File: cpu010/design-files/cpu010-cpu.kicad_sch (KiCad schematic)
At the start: 3 parts, among them U201 MC68010P, U202 74ACT163, Y201 40MHz

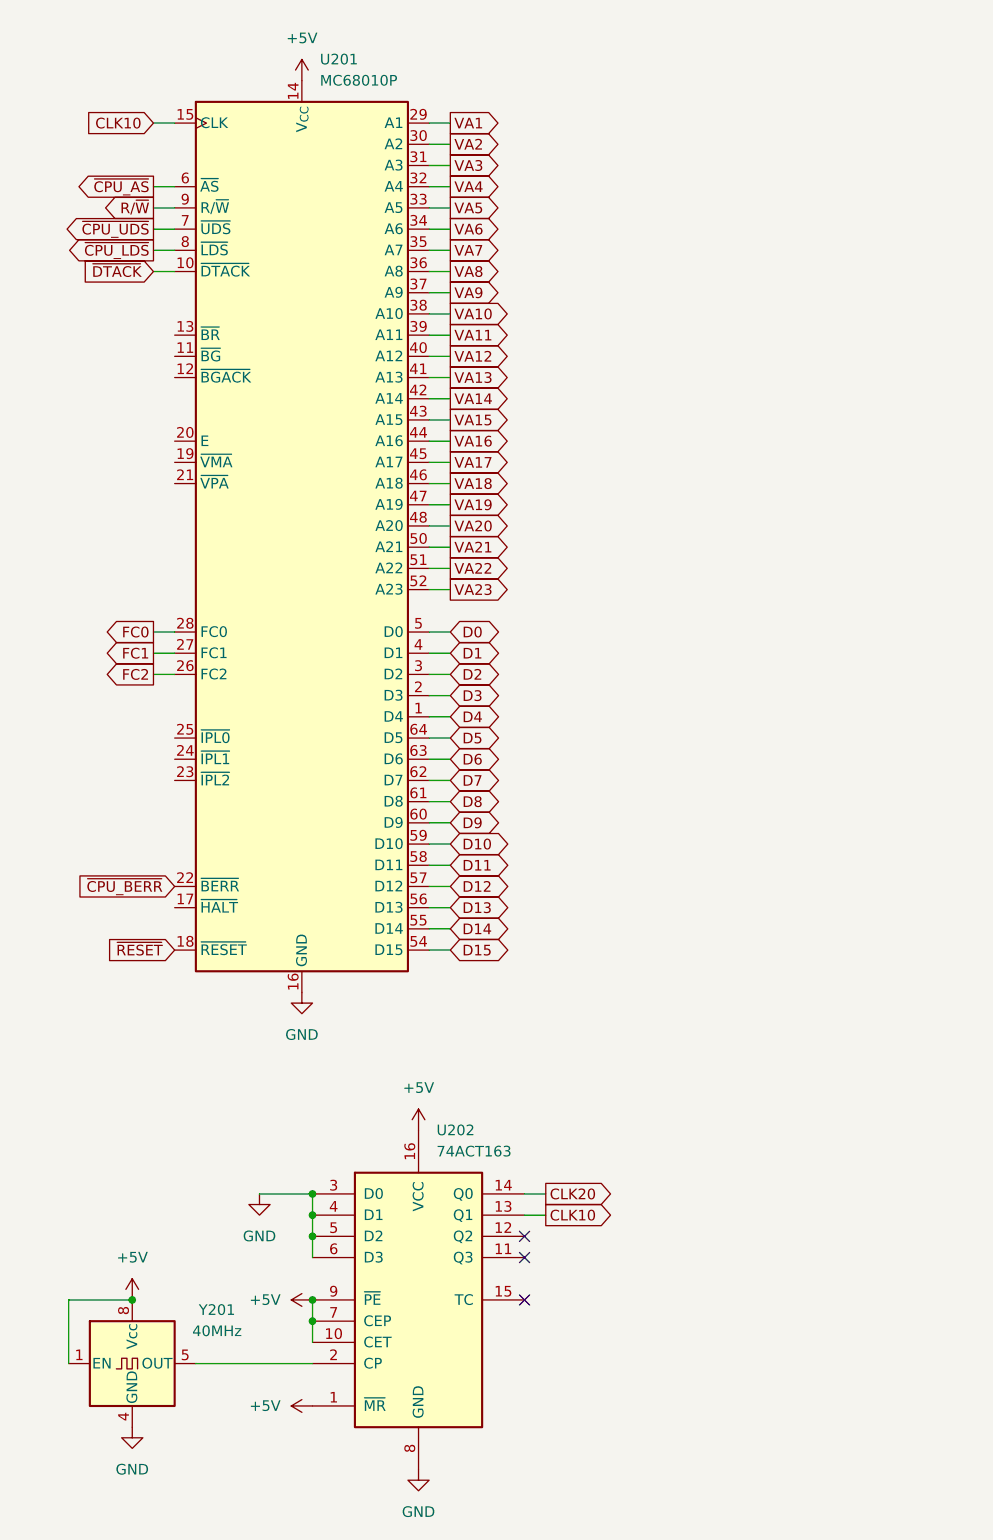
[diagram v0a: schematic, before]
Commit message: Open-drain inverter for DTACKs.
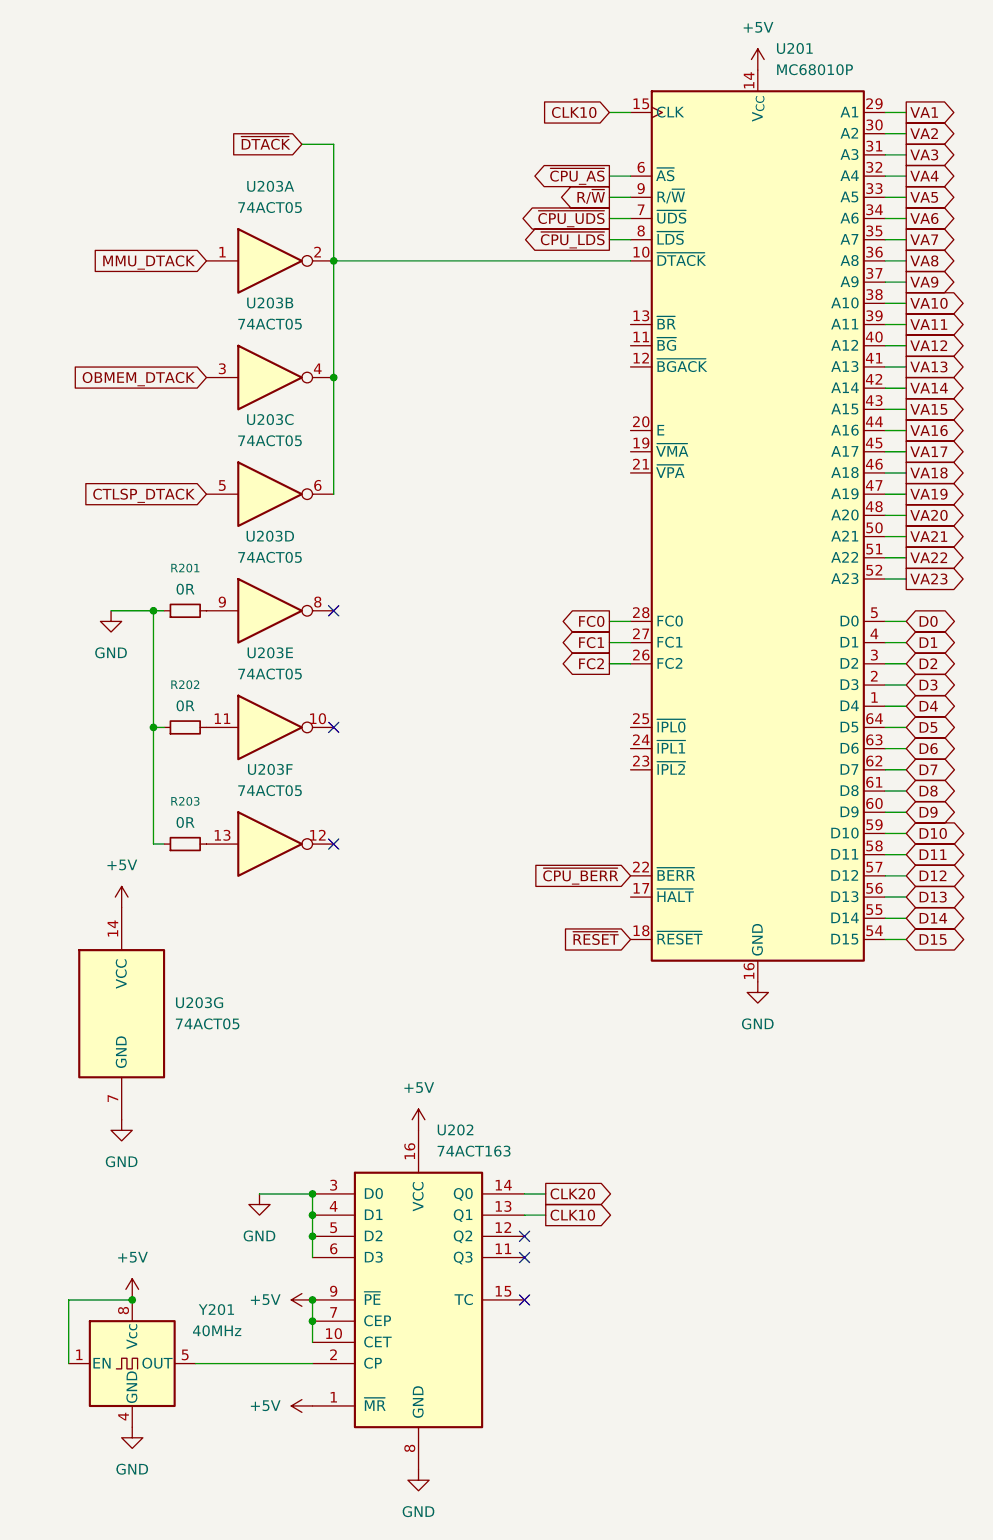
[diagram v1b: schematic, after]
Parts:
- added R201, R202, R203: 0R, Resistor_THT:R_Axial_DIN0207_L6.3mm_D2.5mm_P7.62mm_Horizontal, symbol Device:R_Small
- added U203: 74ACT05, Package_DIP:DIP-14_W7.62mm_Socket, symbol 74xx:74LS05
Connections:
- net +5V: now also U203.14 (VCC)
- net GND: now also R201.1, R202.1, R203.1, U203.7 (GND)
- net ~{DTACK}: now also U203.2, U203.4, U203.6
- new net: R201.2, U203.9
- new net: R202.2, U203.11
- new net: R203.2, U203.13
- new net CTLSP_DTACK: U203.5
- new net MMU_DTACK: U203.1
- new net OBMEM_DTACK: U203.3
- no-connect marks 3 -> 6
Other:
- moved on the sheet: U201
